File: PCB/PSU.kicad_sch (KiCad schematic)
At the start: 21 parts, among them Q1 2N7002, U1 AMS1117-3.3, U6 AP2127K-ADJ, U8 TUSB320LA, U9 TPS2557

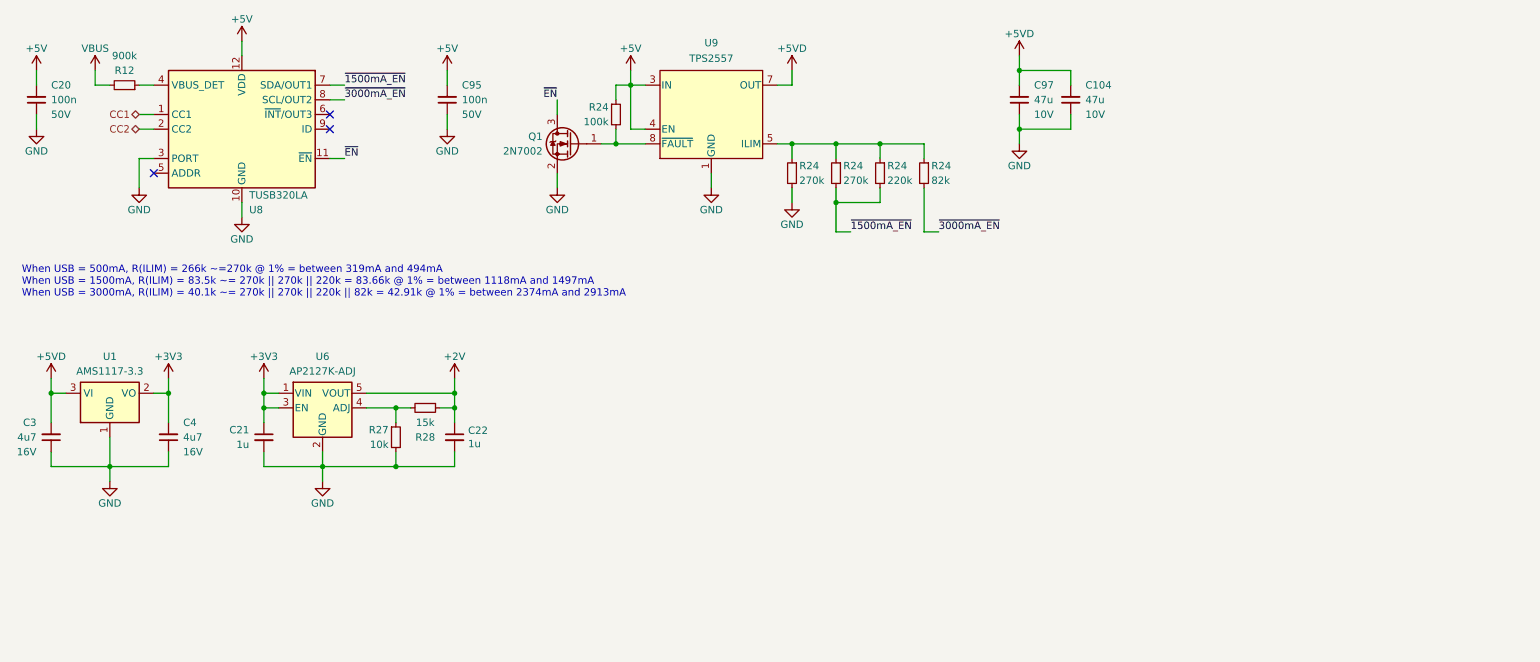
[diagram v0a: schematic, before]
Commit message: 17/04/2023 large update.
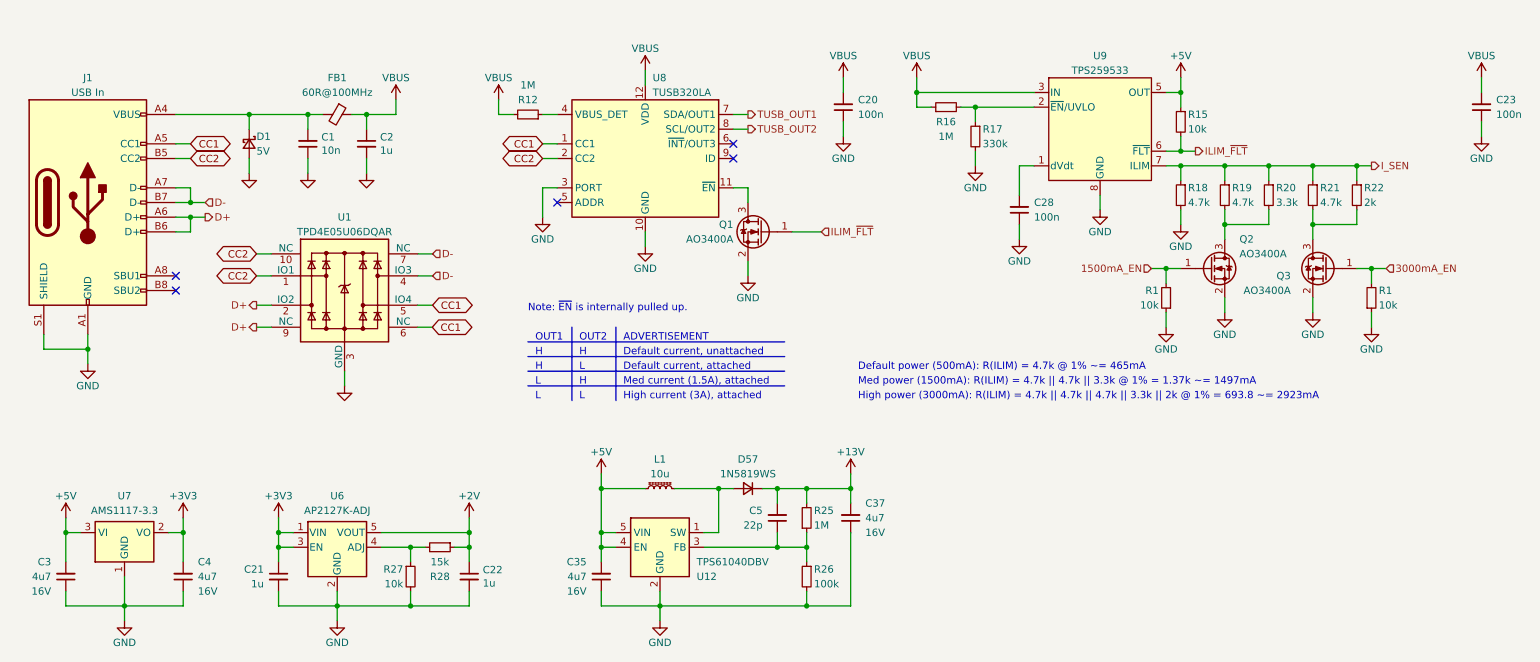
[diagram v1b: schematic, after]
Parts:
- removed C104, C97: 47u, Capacitor_SMD:C_1206_3216Metric, symbol Device:C_Small
- removed C95: 100n, Capacitor_SMD:C_0402_1005Metric, symbol Device:C_Small
- removed Q1: 2N7002, Package_TO_SOT_SMD:SOT-23, symbol Transistor_FET:2N7002
- removed R24 (x2): 270k, Resistor_SMD:R_0402_1005Metric, symbol Device:R_Small
- removed R24: 82k, Resistor_SMD:R_0402_1005Metric, symbol Device:R_Small
- removed R24: 220k, Resistor_SMD:R_0402_1005Metric, symbol Device:R_Small
- removed R24: 100k, Resistor_SMD:R_0402_1005Metric, symbol Device:R_Small
- removed U1: AMS1117-3.3, Package_TO_SOT_SMD:SOT-223-3_TabPin2, symbol Regulator_Linear:AMS1117-3.3
- removed U9: TPS2557, Honeydew:HVSON-8-1EP_3x3mm_P0.65mm_EP1.6x2.4mm, symbol Honeydew:TPS2557
- added C1: 10n, Capacitor_SMD:C_0402_1005Metric, symbol Device:C_Small
- added C2: 1u, Capacitor_SMD:C_0603_1608Metric, symbol Device:C_Small
- added C23, C28: 100n, Capacitor_SMD:C_0402_1005Metric, symbol Device:C_Small
- added C35, C37: 4u7, Capacitor_SMD:C_0603_1608Metric, symbol Device:C_Small
- added C5: 22p, Capacitor_SMD:C_0402_1005Metric, symbol Device:C_Small
- added D1: 5V, Diode_SMD:D_SOD-523, symbol Device:D_Schottky_Small
- added D57: 1N5819WS, Diode_SMD:D_SOD-323, symbol Device:D_Small
- added FB1: 60R@100MHz, Inductor_SMD:L_0805_2012Metric, symbol Device:FerriteBead_Small
- added J1: USB In, Honeydew:HRO-TYPE-C-31-M-13x, symbol Connector:USB_C_Receptacle_USB2.0
- added L1: 10u, Inductor_SMD:L_Sunlord_SWPA3012S, symbol Device:L_Ferrite_Small
- added Q1, Q2, Q3: AO3400A, Package_TO_SOT_SMD:SOT-23, symbol Transistor_FET:AO3400A
- added R1 (x2), R15: 10k, Resistor_SMD:R_0402_1005Metric, symbol Device:R_Small
- added R16, R25: 1M, Resistor_SMD:R_0402_1005Metric, symbol Device:R_Small
- added R17: 330k, Resistor_SMD:R_0402_1005Metric, symbol Device:R_Small
- added R18, R19, R21: 4.7k, Resistor_SMD:R_0402_1005Metric, symbol Device:R_Small
- added R20: 3.3k, Resistor_SMD:R_0402_1005Metric, symbol Device:R_Small
- added R22: 2k, Resistor_SMD:R_0402_1005Metric, symbol Device:R_Small
- added R26: 100k, Resistor_SMD:R_0402_1005Metric, symbol Device:R_Small
- added U1: TPD4E05U06DQAR, Honeydew:USON-10_2.5x1.0mm_P0.5mm, symbol Casaba:TPD4E05U06DQAR
- added U12: TPS61040DBV, Package_TO_SOT_SMD:SOT-23-5, symbol Regulator_Switching:TPS61040DBV
- added U7: AMS1117-3.3, Package_TO_SOT_SMD:SOT-223-3_TabPin2, symbol Regulator_Linear:AMS1117-3.3
- added U9: TPS259533, Honeydew:WSON-8-1EP_2x2mm_P0.5mm_EP0.9x1.6mm, symbol Honeydew:TPS259533
- R12: value 900k -> 1M; LCSC C25905 -> C26083
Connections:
- net +5VD is gone; now on net +5V: C3.2
- net +3V3: now also U7.2 (VO)
- net +5V: now also C35.2, L1.2, R15.1, U12.4 (EN), U12.5 (VIN), U7.3 (VI), U9.5 (OUT); no longer C20.2, U8.12 (VDD)
- net CC1: now also J1.A5 (CC1), U1.5 (IO4), U1.6 (NC)
- net CC2: now also J1.B5 (CC2), U1.1 (IO1), U1.10 (NC)
- net GND: now also C1.1, C2.2, C23.1, C28.1, C35.1, C37.1, D1.2 (A), J1.A1 (GND), J1.A12 (GND), J1.B1 (GND), J1.B12 (GND), J1.S1 (SHIELD), Q1.2 (S), Q2.2 (S), Q3.2 (S), R1.1, R1.1, R17.2, R18.2, R26.2, U1.3 (GND), U1.8 (GND), U12.2 (GND), U7.1 (GND), U9.8 (GND), U9.9 (GND)
- net VBUS renamed IN
- net IN: now also C20.2, U8.12 (VDD), C2.1, C23.2, FB1.1, R16.1, U9.3 (IN), U9.4 (IN)
- net ~{1500mA_EN} renamed TUSB_OUT1
- net ~{3000mA_EN} renamed TUSB_OUT2
- net ~{EN}: no longer names the net of U8.11 (~{EN})
- net ~{EN}: now also Q1.3 (D)
- new net: C5.1, R25.1, R26.1, U12.3 (FB)
- new net: Q2.3 (D), R19.2, R20.2
- new net: D57.2 (A), L1.1, U12.1 (SW)
- new net: Q3.3 (D), R21.2, R22.2
- new net: C1.2, D1.1 (K), FB1.2, J1.A4 (VBUS), J1.A9 (VBUS), J1.B4 (VBUS), J1.B9 (VBUS)
- new net: C28.2, U9.1 (dVdt)
- new net: R16.2, R17.1, U9.2 (~{EN}/UVLO)
- new net +13V: C37.2, C5.2, D57.1 (K), R25.2
- new net 1500mA_EN: Q2.1 (G), R1.2
- new net 3000mA_EN: Q3.1 (G), R1.2
- new net D+: J1.A6 (D+), J1.B6 (D+), U1.2 (IO2), U1.9 (NC)
- new net D-: J1.A7 (D-), J1.B7 (D-), U1.4 (IO3), U1.7 (NC)
- new net ILIM_~{FLT}: Q1.1 (G), R15.2, U9.6 (~{FLT})
- new net I_SEN: R18.1, R19.1, R20.1, R21.1, R22.1, U9.7 (ILIM)
- no-connect marks 3 -> 5
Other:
- note added: "ADVERTISEMENT"
- note added: "Default current, attached"
- note added: "Default current, unattached"
- note added: "Default power (500mA): R(ILIM) = 4.7k @ 1% ~= 465mA"
- note added: "H"
- note added: "High current (3A), attached"
- note added: "High power (3000mA): R(ILIM) = 4.7k || 4.7k || 4.7k || 3.3k || 2k @ 1% = 693.8 ~= 2923mA"
- note added: "L"
- note added: "Med current (1.5A), attached"
- note added: "Med power (1500mA): R(ILIM) = 4.7k || 4.7k || 3.3k @ 1% = 1.37k ~= 1497mA"
- note added: "Note: ~{EN} is internally pulled up."
- note added: "OUT1"
- note added: "OUT2"
- note removed: "When USB = 500mA, R(ILIM) = 266k ~=270k @ 1% = between 319mA and 494mA When USB = 1500mA, R(ILIM) = 83.5k ~= 270k || 270k || 220k = 83.66k @ 1% = between 1118mA and 1497mA When USB = 3000mA, R(ILIM) = 40.1k ~= 270k || 270k || 220k || 82k = 42.91k @ 1% = between 2374mA and 2913mA"
- moved on the sheet: C20, C21, C22, C3, C4, R12, R27, R28, U6, U8
